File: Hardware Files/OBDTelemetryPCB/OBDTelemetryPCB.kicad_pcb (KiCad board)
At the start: 2 copper layers, 50 x 38 mm, 5 parts, among them J1 InputSocket, U1 ESP32-WROOM-32E, U2 SN65HVD230, U3 CP2102N-Axx-xQFN24, U4 TLV76133DCY

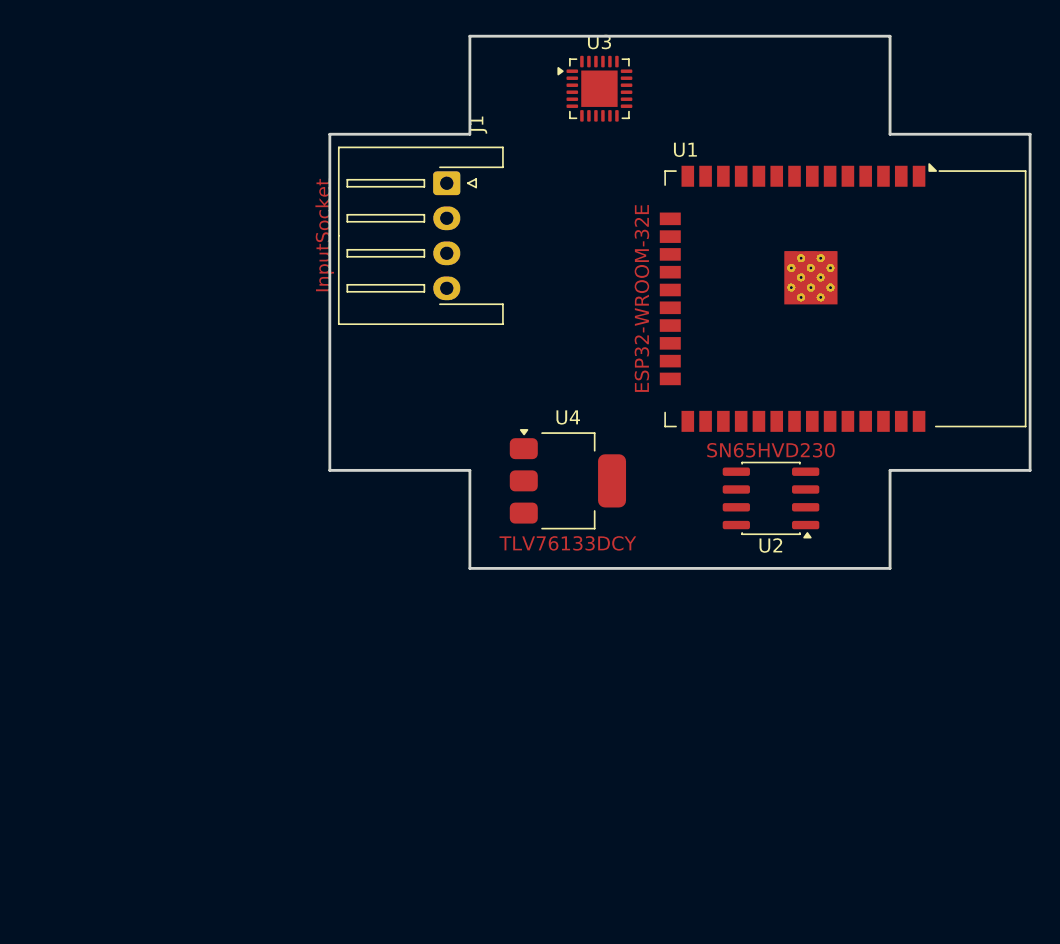
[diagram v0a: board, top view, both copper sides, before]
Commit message: Completed v1 of hardware
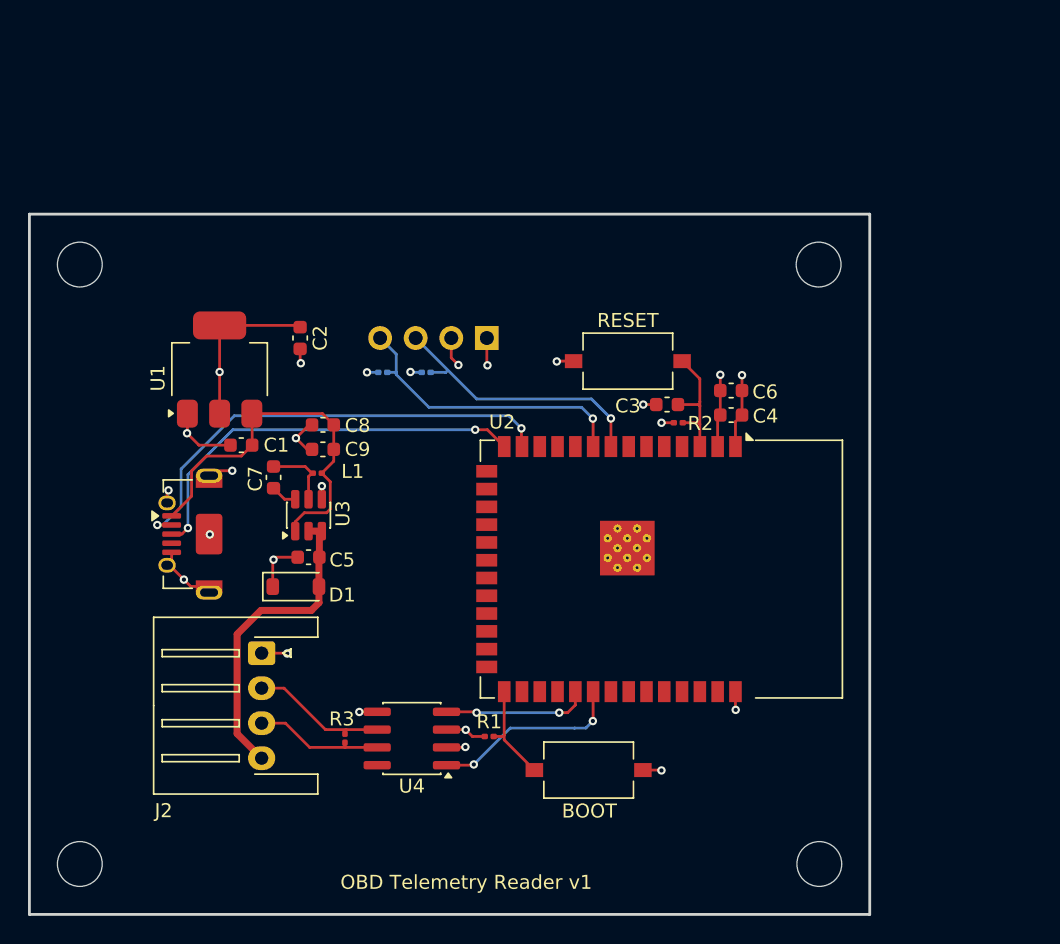
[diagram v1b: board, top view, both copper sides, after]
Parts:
- removed the U1 at (159.8, 84.5)
- added C1: 1uF, Capacitor_SMD:C_0603_1608Metric, F.Cu at (119.7, 95.0)
- added C2: 2.2uF, Capacitor_SMD:C_0603_1608Metric, F.Cu at (123.9, 87.3)
- added C3: 1uF, Capacitor_SMD:C_0603_1608Metric, F.Cu at (150.1, 92.0)
- added C4: 0.1uF, Capacitor_SMD:C_0603_1608Metric, F.Cu at (154.7, 92.8)
- added C5: 10uF, Capacitor_SMD:C_0603_1608Metric, F.Cu at (124.5, 103.0)
- added C6: 10uF, Capacitor_SMD:C_0603_1608Metric, F.Cu at (154.7, 91.0)
- added C7: 100nF, Capacitor_SMD:C_0603_1608Metric, F.Cu at (122.0, 97.2)
- added C8: 22uF, Capacitor_SMD:C_0603_1608Metric, F.Cu at (125.5, 93.5)
- added C9: 22uF, Capacitor_SMD:C_0603_1608Metric, F.Cu at (125.5, 95.2)
- added D1: SM6T15A, Diode_SMD:D_SOD-123, F.Cu at (123.6, 105.0)
- added J1: USB_B_Micro, Connector_USB:USB_Micro-AB_Molex_47590-0001, F.Cu at (117.7, 101.3)
- added J3: Conn_01x04_Socket, Connector_PinHeader_2.54mm:PinHeader_1x04_P2.54mm_Vertical, B.Cu at (137.2, 87.3)
- added L1: 4.7uH, Resistor_SMD:R_0201_0603Metric, F.Cu at (125.1, 97.0)
- added R1: 10k, Resistor_SMD:R_0201_0603Metric, F.Cu at (137.4, 115.8)
- added R2: 10k, Resistor_SMD:R_0201_0603Metric, F.Cu at (150.9, 93.3)
- added R3: 120, Resistor_SMD:R_0201_0603Metric, F.Cu at (127.1, 115.9)
- added R4: 4.7k, Resistor_SMD:R_0201_0603Metric, B.Cu at (129.8, 89.8)
- added R5: 4.7k, Resistor_SMD:R_0201_0603Metric, B.Cu at (132.9, 89.8)
- added REF**: MountingHole_3.2mm_M3, MountingHole:MountingHole_3.2mm_M3, F.Cu at (108.2, 82.1)
- added REF**: MountingHole_3.2mm_M3, MountingHole:MountingHole_3.2mm_M3, F.Cu at (160.9, 82.1)
- added REF**: MountingHole_3.2mm_M3, MountingHole:MountingHole_3.2mm_M3, F.Cu at (108.2, 124.9)
- added REF**: MountingHole_3.2mm_M3, MountingHole:MountingHole_3.2mm_M3, F.Cu at (160.9, 124.9)
- added SW1: BOOT, Button_Switch_SMD:SW_Tactile_SPST_NO_Straight_CK_PTS636Sx25SMTRLFS, F.Cu at (144.5, 118.2)
- added SW2: RESET, Button_Switch_SMD:SW_Tactile_SPST_NO_Straight_CK_PTS636Sx25SMTRLFS, F.Cu at (147.3, 89.0)
- added U2: ESP32-S3-WROOM-1, RF_Module:ESP32-S3-WROOM-1, F.Cu at (149.7, 103.8)
- U3: value CP2102N-Axx-xQFN24 -> AP63205WU; footprint Package_DFN_QFN:QFN-24-1EP_4x4mm_P0.5mm_EP2.6x2.6mm -> Package_TO_SOT_SMD:TSOT-23-6
- moved U3 36.9 mm to (124.5, 100.0), turned to 90 degrees
- moved J2 36.1 mm to (121.1, 109.8)
- moved U4 30.8 mm to (131.9, 115.9)
- moved U1 26.1 mm to (118.1, 89.5), turned to 90 degrees
- renumbered J1 to J2, U4 to U1, U2 to U4
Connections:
- U1 pad 3: +12V -> +5V
- U3 pad 1: unconnected-(U3-~{RI}/CLK-Pad1) -> +5V
- U3 pad 2: GND -> +12V
- U3 pad 3: /D+ -> +12V
- U3 pad 4: /D- -> GND
- U3 pad 5: unconnected-(U3-VIO-Pad5) -> Net-(U3-SW)
- U3 pad 6: +3.3V -> Net-(U3-BST)
- U4 pad 1: /D -> /DTX
- U4 pad 4: /R -> /RTX
- U4 pad 5: unconnected-(U2-Vref-Pad5) -> GND
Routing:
- net GND: track 0.00 -> 37.6 mm, vias 0 -> 18
- net /D-: track 0.00 -> 33.5 mm, vias 0 -> 2
- net /D+: track 0.00 -> 29.6 mm, vias 0 -> 2
- net +5V: track 0.00 -> 27.5 mm
- net +3.3V: track 0.00 -> 24.9 mm, vias 0 -> 7
- net +12V: track 0.34 -> 22.5 mm
- net /SDA: track 0.00 -> 21.1 mm, vias 0 -> 1
- net /SCL: track 0.00 -> 19.6 mm, vias 0 -> 1
- net /DTX: track 0.00 -> 13.9 mm, vias 0 -> 2
- net /RTX: track 0.00 -> 10.6 mm, vias 0 -> 2
- net /CANL: track 0.00 -> 9.80 mm
- net /EN: track 0.00 -> 9.49 mm
- net /CANH: track 0.00 -> 9.30 mm
- net /BOOT: track 0.00 -> 7.78 mm
- net Net-(U3-SW): track 0.00 -> 4.90 mm
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- added copper zone on In1.Cu, net +3.3V
- added copper zone on In2.Cu, net GND
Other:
- board size 50 x 38 mm -> 60 x 50 mm
- copper layers 2 -> 4
- board text added: "OBD Telemetry Reader v1"
